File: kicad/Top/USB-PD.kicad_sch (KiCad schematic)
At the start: 33 parts, among them J6 M20-9990246, Q6 SI4477DY-T1-GE3, Q7 SI4477DY-T1-GE3

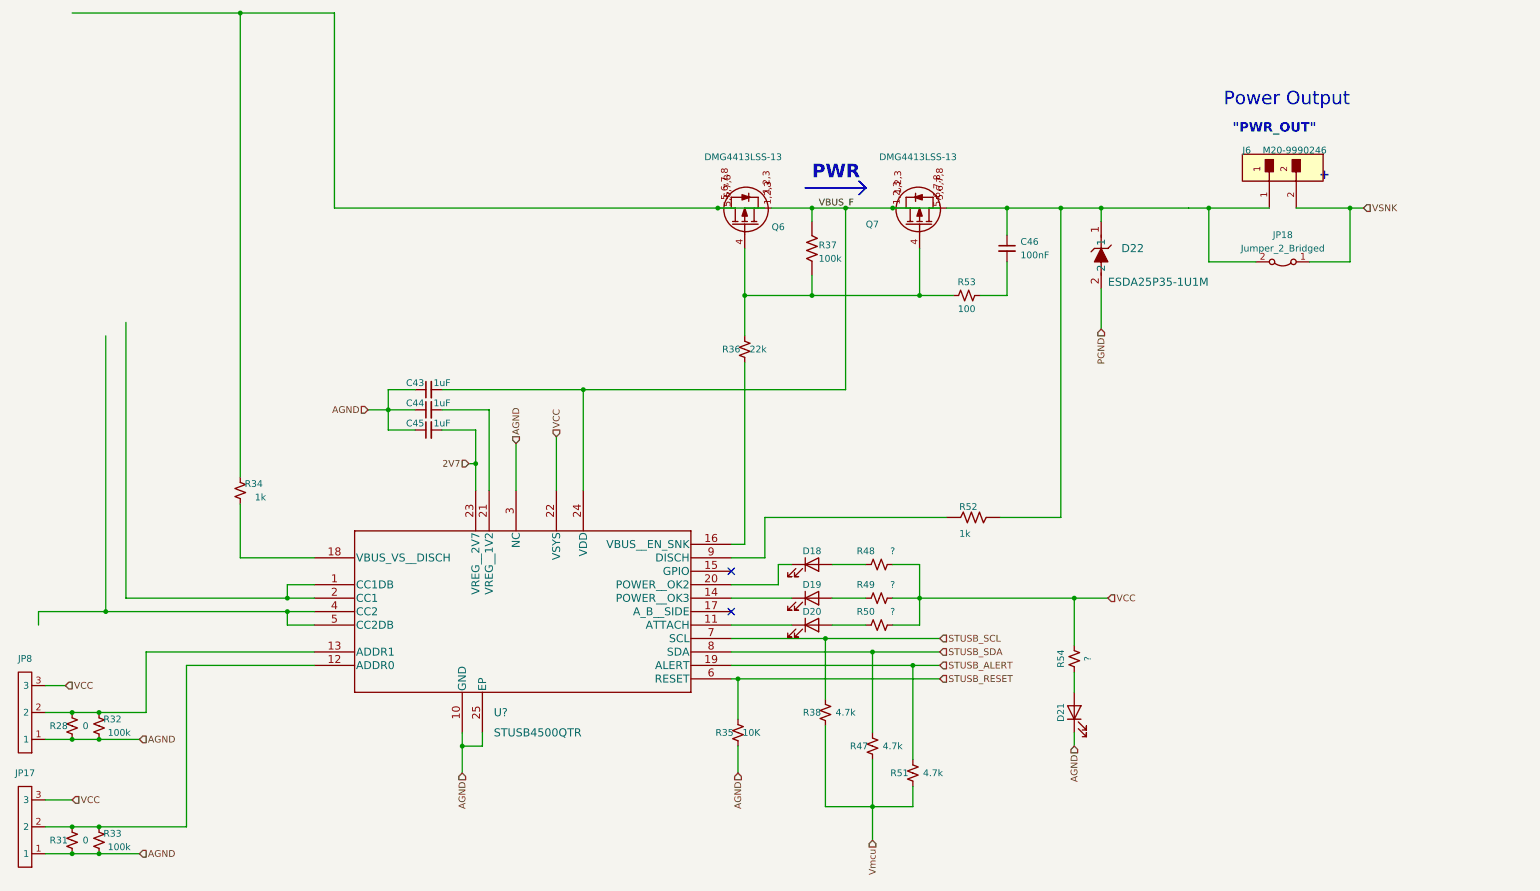
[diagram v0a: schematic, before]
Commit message: wip started working on pd sheet but need more info before proceeding
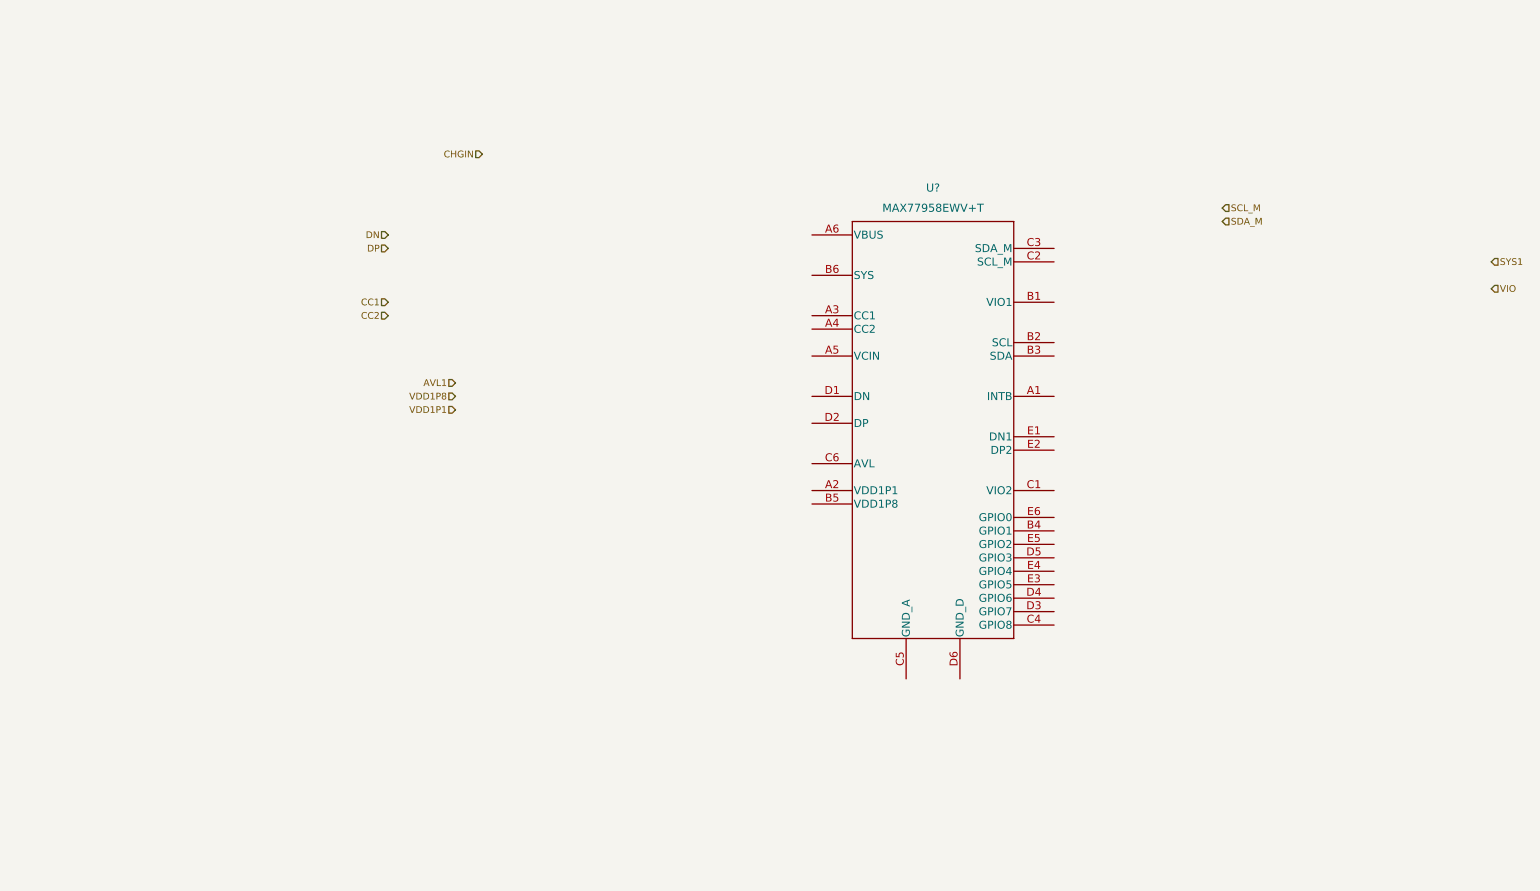
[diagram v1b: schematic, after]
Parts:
- removed C43, C44, C45: 1uF, symbol Device:C_Small
- removed C46: 100nF, symbol Device:C_Small
- removed D18, D19, D20, D21: LED, symbol Device:LED
- removed D22: ESDA25P35-1U1M, custom_modules:ESDA25P35-1U1M, symbol ESDA25P35-1U1M:ESDA25P35-1U1M
- removed J6: M20-9990246, AltiumImports:FP-M20-9990246-MFG, symbol Top-altium-import:3_mirrored_3bc925449376181038e59eaffc5286c
- removed JP17, JP8: 3-pad-selection, symbol custom_connectors:3-pad-selection
- removed JP18: Jumper_2_Bridged, symbol Jumper:Jumper_2_Bridged
- removed Q6: SI4477DY-T1-GE3, AltiumImports:_ALTIUM_WORK_00001_MCHP-CDB_Library_Database_.._Footprints_SOIC-8.PcbLib_SOIC-8, symbol Top-altium-import:1_mirrored_SI4477DY-T1-GE3
- removed Q7: SI4477DY-T1-GE3, AltiumImports:_ALTIUM_WORK_00001_MCHP-CDB_Library_Database_.._Footprints_SOIC-8.PcbLib_SOIC-8, symbol Top-altium-import:1_SI4477DY-T1-GE3
- removed R28, R31: 0, symbol Device:R_Small_US
- removed R32, R33: 100k, symbol Device:R_Small_US
- removed R34: 1k, symbol Device:R_Small_US
- removed R35: 10K, symbol Device:R_Small_US
- removed R36: 22k, symbol Device:R_Small_US
- removed R37: Resistor, AltiumImports:_ALTIUM_WORK_00001_MCHP-CDB_Library_Database_.._Footprints_RES_C_0402.PcbLib_RES_C_0402, symbol Top-altium-import:1_Resistor
- removed R38, R47, R51: 4.7k, symbol Device:R_Small_US
- removed R48, R49, R50, R54: ?, symbol Device:R_Small_US
- removed R52: Resistor, AltiumImports:_ALTIUM_WORK_00001_MCHP-CDB_Library_Database_.._Footprints_RES_C_0402.PcbLib_RES_C_0402, symbol Top-altium-import:0_Resistor
- removed R53: 100, symbol Device:R_Small_US
- removed U?: STUSB4500QTR, Ultra_Librarian:QFN24EP_4X4_STM, symbol ultralibrarian:STUSB4500QTR
- added U?: MAX77958EWV+T, Ultra_Librarian:MAX77958EWV&plus_T, symbol ultralibrarian:MAX77958EWV+T
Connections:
- no-connect marks 2 -> 0
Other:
- note removed: ""PWR_OUT""
- note removed: "+"
- note removed: "PWR"
- note removed: "Power Output"
